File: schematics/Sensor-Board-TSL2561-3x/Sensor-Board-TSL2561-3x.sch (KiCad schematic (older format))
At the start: 10 parts, among them P1 CONN_02X04, U1 TSL2561, U2 TSL2561, U3 TSL2561

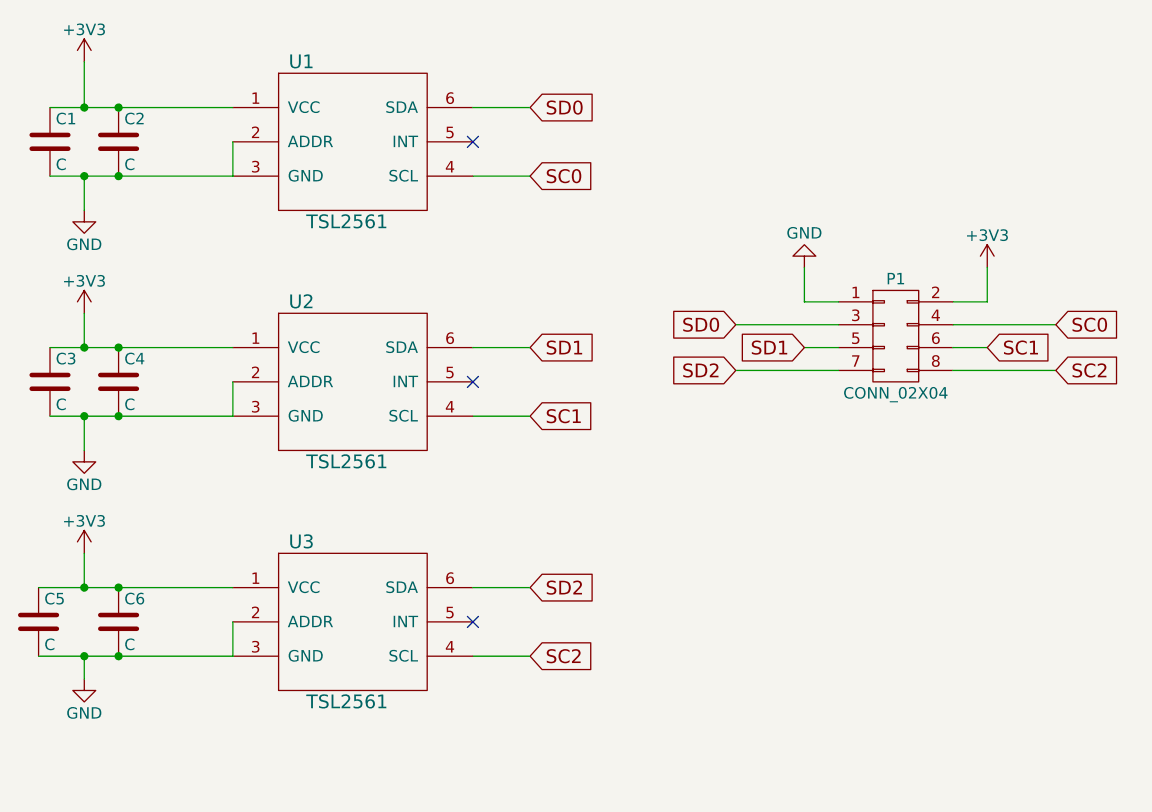
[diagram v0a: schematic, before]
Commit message: Schematics update
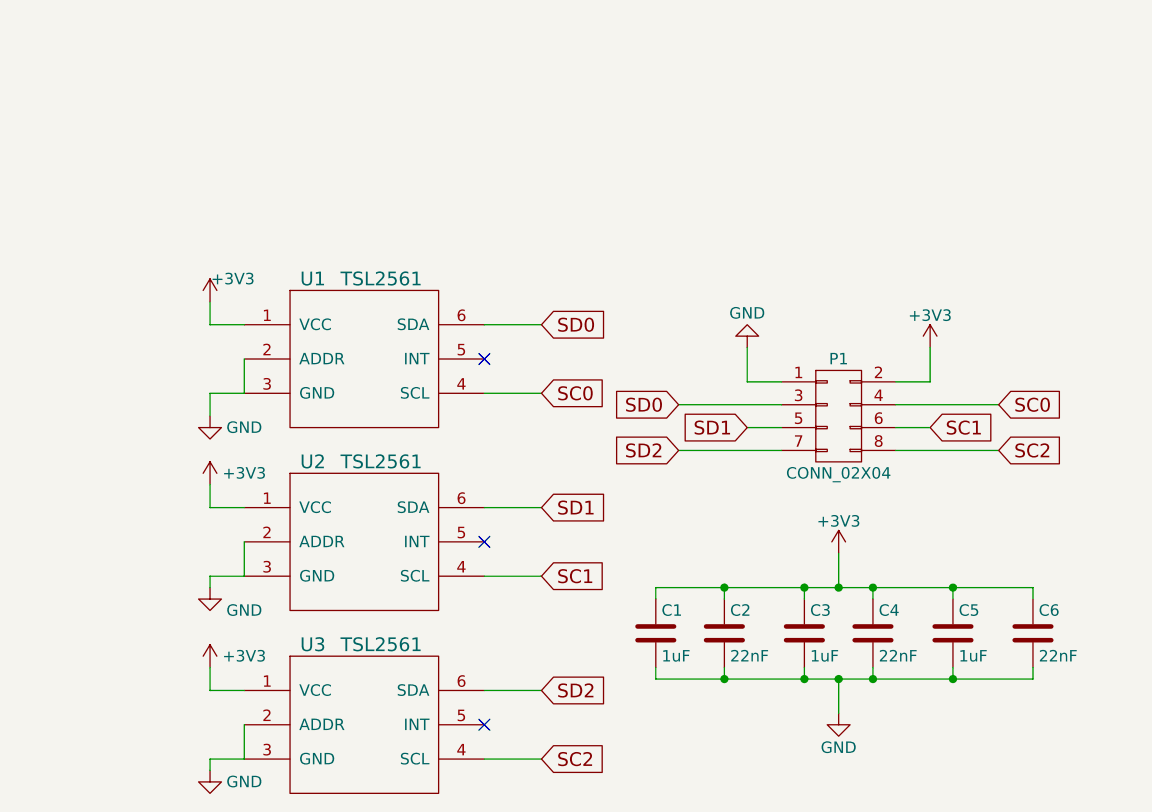
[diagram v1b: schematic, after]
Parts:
- C1, C3, C5: value C -> 1uF
- C2, C4, C6: value C -> 22nF
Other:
- moved on the sheet: C1, C2, C3, C4, C5, C6, P1, U1, U2, U3
